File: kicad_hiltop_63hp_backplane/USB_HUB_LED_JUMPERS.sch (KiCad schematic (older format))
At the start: 81 parts, among them J12 4POS_JUMPER, J13 4POS_JUMPER, J14 4POS_JUMPER, J15 4POS_JUMPER, J16 4POS_JUMPER, U5 USB2517, Y2 24Mhz Xtal

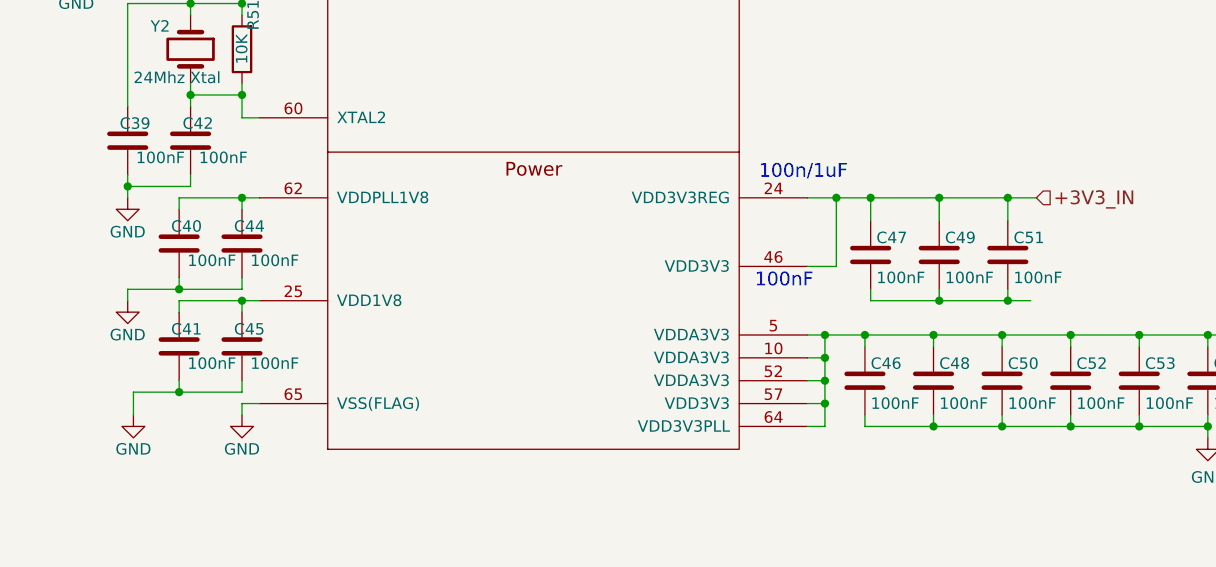
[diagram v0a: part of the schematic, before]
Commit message: first pass schematic placement
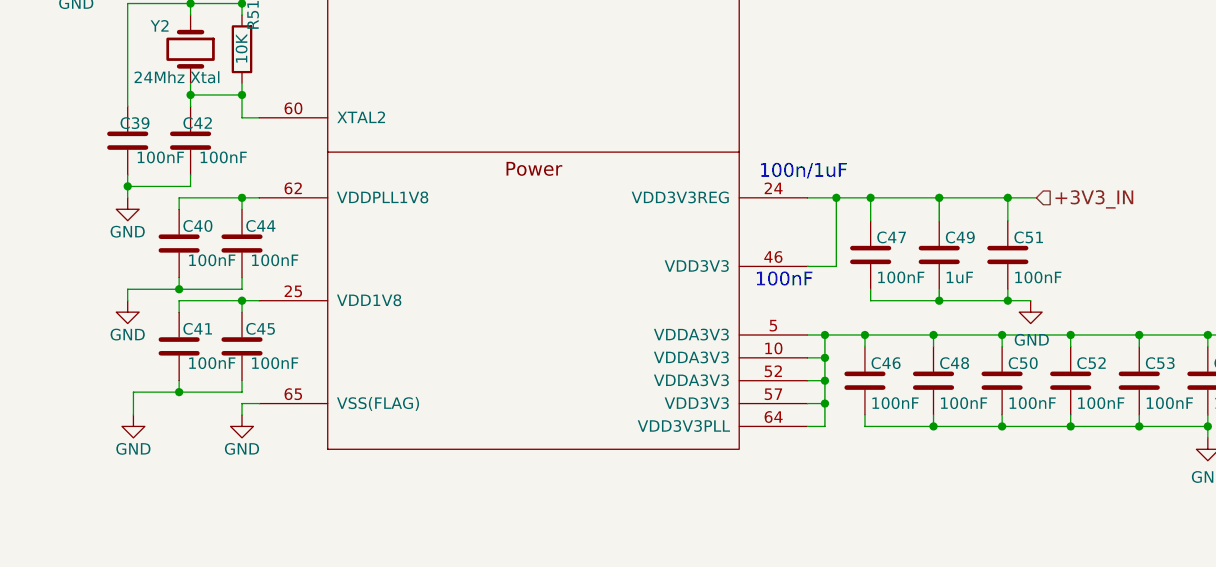
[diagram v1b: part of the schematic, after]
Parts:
- C49: value 100nF -> 1uF
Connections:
- net GND: now also C47.1, C49.1, C51.1
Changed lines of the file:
@@
 $Descr A4 11693 8268
 encoding utf-8
-Sheet 6 6
+Sheet 5 6
 Title ""
 Date ""
@@
 P 5375 4150
 F 0 "C49" H 5350 4075 50  0000 R CNN
-F 1 "100nF" H 5350 4250 50  0000 R CNN
+F 1 "1uF" H 5350 4250 50  0000 R CNN
 F 2 "Capacitor_SMD:C_0603_1608Metric" H 5413 4000 50  0001 C CNN
 F 3 "" H 5375 4150 50  0001 C CNN
@@
 AR Path="/5A077B59/5CBF7F97" Ref="C?"  Part="1"
 AR Path="/5A077C30/5CBF7F97" Ref="C40"  Part="1"
-F 0 "C40" H 1950 4025 50  0000 L CNN
+F 0 "C40" H 1900 4025 50  0000 L CNN
 F 1 "100nF" H 1800 4175 50  0000 L CNN
 F 2 "Capacitor_SMD:C_0603_1608Metric" H 2088 3950 50  0001 C CNN
@@
 AR Path="/5A077B59/5CBF8081" Ref="C?"  Part="1"
 AR Path="/5A077C30/5CBF8081" Ref="C44"  Part="1"
-F 0 "C44" H 2225 4025 50  0000 L CNN
+F 0 "C44" H 2175 4025 50  0000 L CNN
 F 1 "100nF" H 2075 4175 50  0000 L CNN
 F 2 "Capacitor_SMD:C_0603_1608Metric" H 2363 3950 50  0001 C CNN
@@
 AR Path="/5A077B59/5CBF82F9" Ref="C?"  Part="1"
 AR Path="/5A077C30/5CBF82F9" Ref="C41"  Part="1"
-F 0 "C41" H 1950 4475 50  0000 L CNN
+F 0 "C41" H 1900 4475 50  0000 L CNN
 F 1 "100nF" H 1800 4625 50  0000 L CNN
 F 2 "Capacitor_SMD:C_0603_1608Metric" H 2088 4400 50  0001 C CNN
@@
 AR Path="/5A077B59/5CBF83E1" Ref="C?"  Part="1"
 AR Path="/5A077C30/5CBF83E1" Ref="C45"  Part="1"
-F 0 "C45" H 2225 4475 50  0000 L CNN
+F 0 "C45" H 2175 4475 50  0000 L CNN
 F 1 "100nF" H 2075 4625 50  0000 L CNN
 F 2 "Capacitor_SMD:C_0603_1608Metric" H 2363 4400 50  0001 C CNN
@@
 NoConn ~ 9750 4125
 NoConn ~ 9750 4725
+$Comp
+L power:GND #PWR?
+U 1 1 5C67A6C1
+P 5775 4350
+F 0 "#PWR?" H 5775 4100 50  0001 C CNN
+F 1 "GND" H 5780 4177 50  0000 C CNN
+F 2 "" H 5775 4350 50  0001 C CNN
+F 3 "" H 5775 4350 50  0001 C CNN
+	1    5775 4350
+	1    0    0    -1
+$EndComp
 $EndSCHEMATC
